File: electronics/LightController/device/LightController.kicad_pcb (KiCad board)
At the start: 2 copper layers, 61.1 x 50.9 mm, 24 parts, among them J1 RF_TX, J2 AC, J3 SERIAL, J4 ICSP, SW1 RotaryEncoder_Switch, SW2 RotaryEncoder_Switch, SW3 RotaryEncoder_Switch, U1 ATMEGA328P-AU, U2 5V07 Transformer, Y1 16MHz

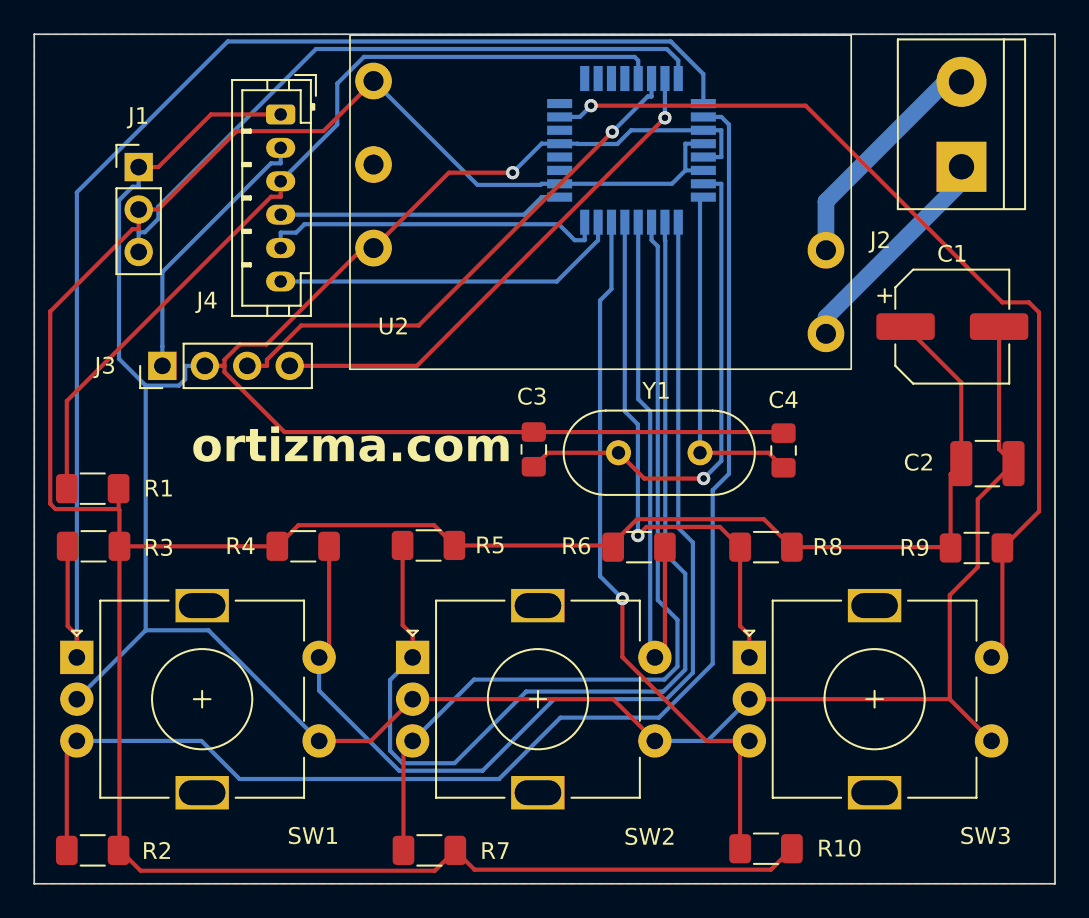
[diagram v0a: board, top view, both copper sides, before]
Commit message: Small adjustments before JLC order
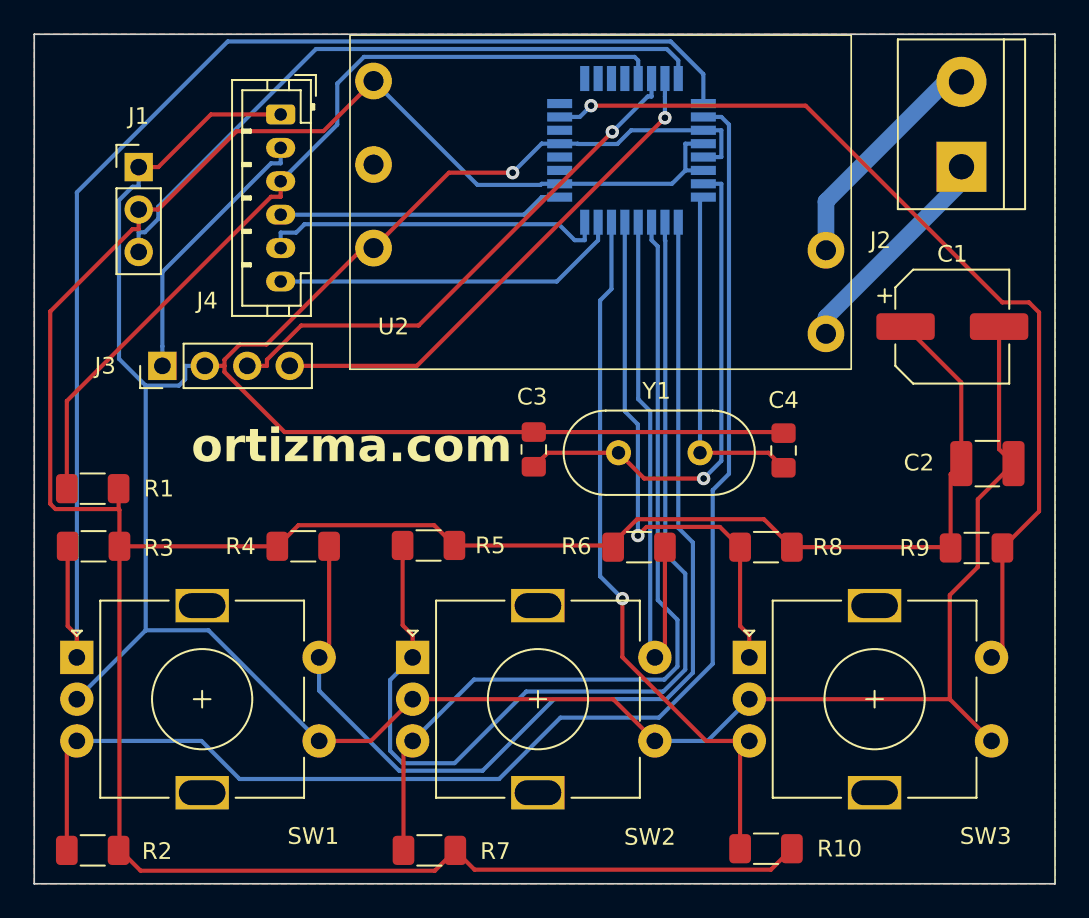
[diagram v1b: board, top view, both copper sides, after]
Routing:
- added copper zone on B.Cu, net GND
